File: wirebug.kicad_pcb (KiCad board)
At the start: 2 copper layers, 35 x 65 mm, 12 parts, among them J1 Screw_Terminal_01x02, J2 Screw_Terminal_01x02, J3 Screw_Terminal_01x02, K1 AW3211F, Q1 BC337, Q2 BC337

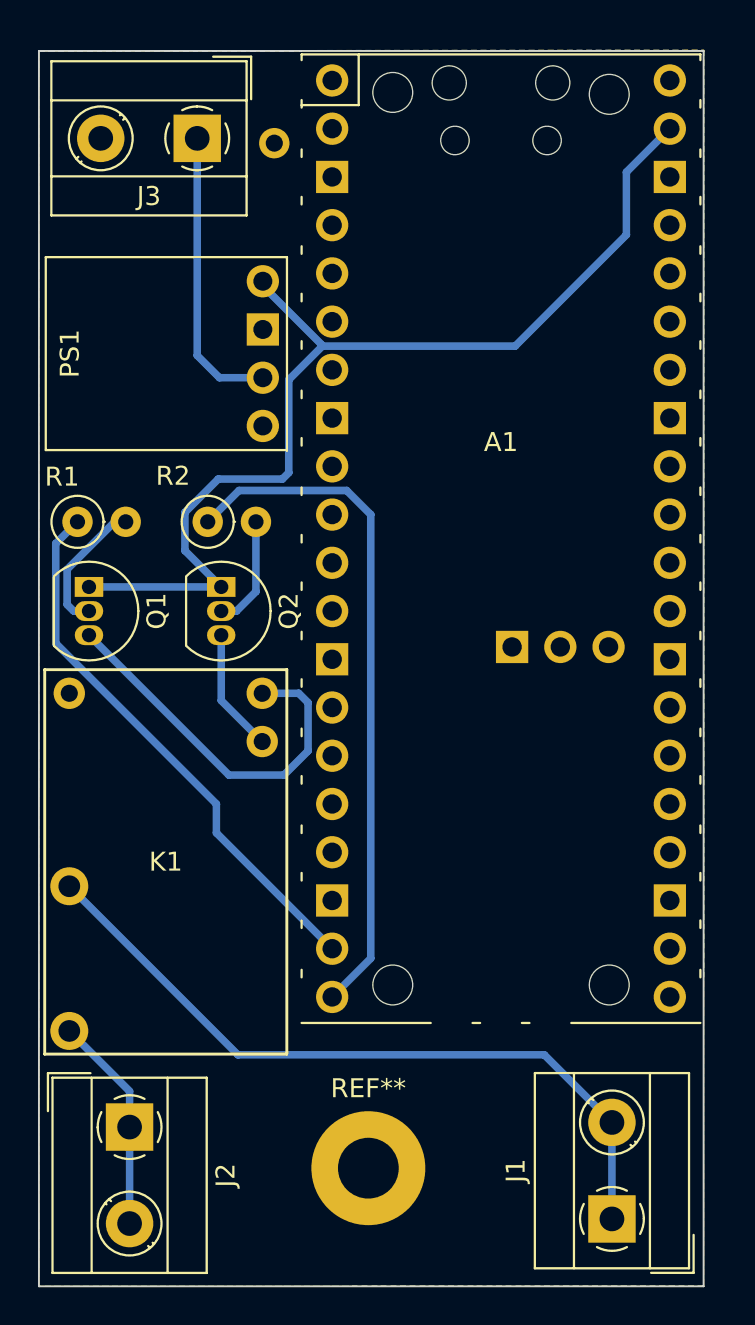
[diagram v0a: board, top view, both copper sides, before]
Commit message: Smaller changes
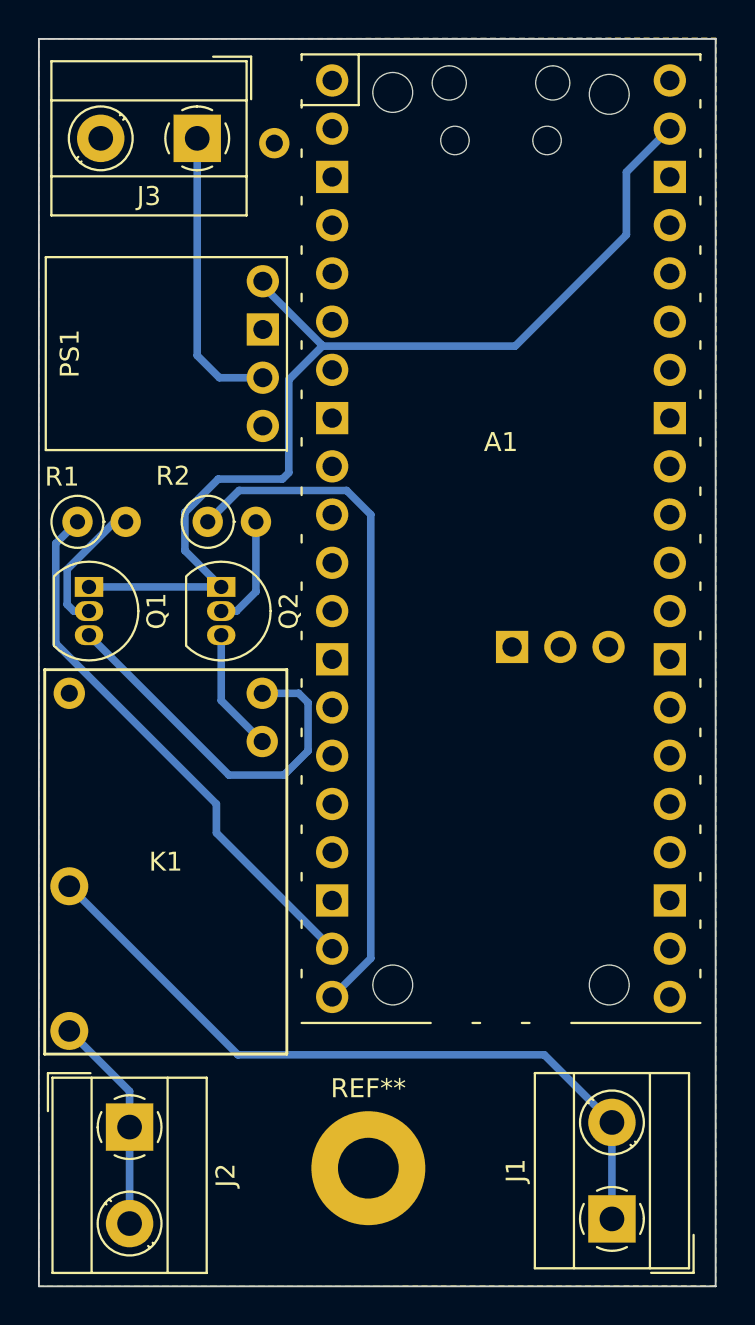
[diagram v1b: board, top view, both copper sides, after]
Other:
- board size 35 x 65 mm -> 35.6 x 65.7 mm
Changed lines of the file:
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@@
     )
   )
-  (gr_rect (start 108.256 50.772) (end 143.256 115.8214)
+  (gr_rect (start 108.256 50.137) (end 143.891 115.8214)
     (stroke (width 0.1) (type default)) (fill none) (layer "Edge.Cuts"))
   (segment (start 134.869 103.632) (end 138.43 107.193) (width 0.4) (layer "B.Cu") (net 3))
@@
     (polygon
       (pts
-        (xy 108.2548 50.7746)
-        (xy 143.2814 50.7238)
-        (xy 143.256 115.7986)
+        (xy 108.2548 50.1396)
+        (xy 143.9164 50.0888)
+        (xy 143.891 115.7986)
         (xy 108.2548 115.824)
       )
